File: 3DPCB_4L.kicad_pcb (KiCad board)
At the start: 4 copper layers, 100 x 60 mm, 758 parts, among them IC1 DRV8825, IC2 DRV8825, IC3 DRV8825, IC4 DRV8825, IC5 DRV8825, IC6 MP9943, J10 , J11 , J12 , J13 , J14 , J15 , J16 , J2 , J3 , J4 , J5 , J6 , J7 , J8 , J9 , K1 CONN_3, K2 CONN_3, K3 CONN_3, K4 CONN_3, K5 CONN_3, K6 CONN_3, K7 CONN_3, K8 CONN_3, K9 CONN_3, P1 CONN_8, P11 CONN_3X2, P12 CONN_3X2, P13 CONN_4, P2 CONN_8, P5 CONN_4, P6 CONN_4, P7 CONN_4, P8 CONN_2, P9 CONN_4, U1 CONN_4_LERCHE, U10 MICRO-SD, U11 IX4427, U12 MCP4728, U13 CONN_4_LERCHE, U15 SPST_MOMENTARY, U16 CONN_4_LERCHE, U17 IX4427, U2 SPST_MOMENTARY, U21 CONN_4_LERCHE, U22 CONN_4_LERCHE, U23 MCP4728, U24 IRFH7932, U25 CONN_4_LERCHE, U3 BSS84, U4 CONN_4_LERCHE, U5 IRFH7932, U6 LPC1768_TQFP100, U7 IRFH7932, U8 IRFH7932

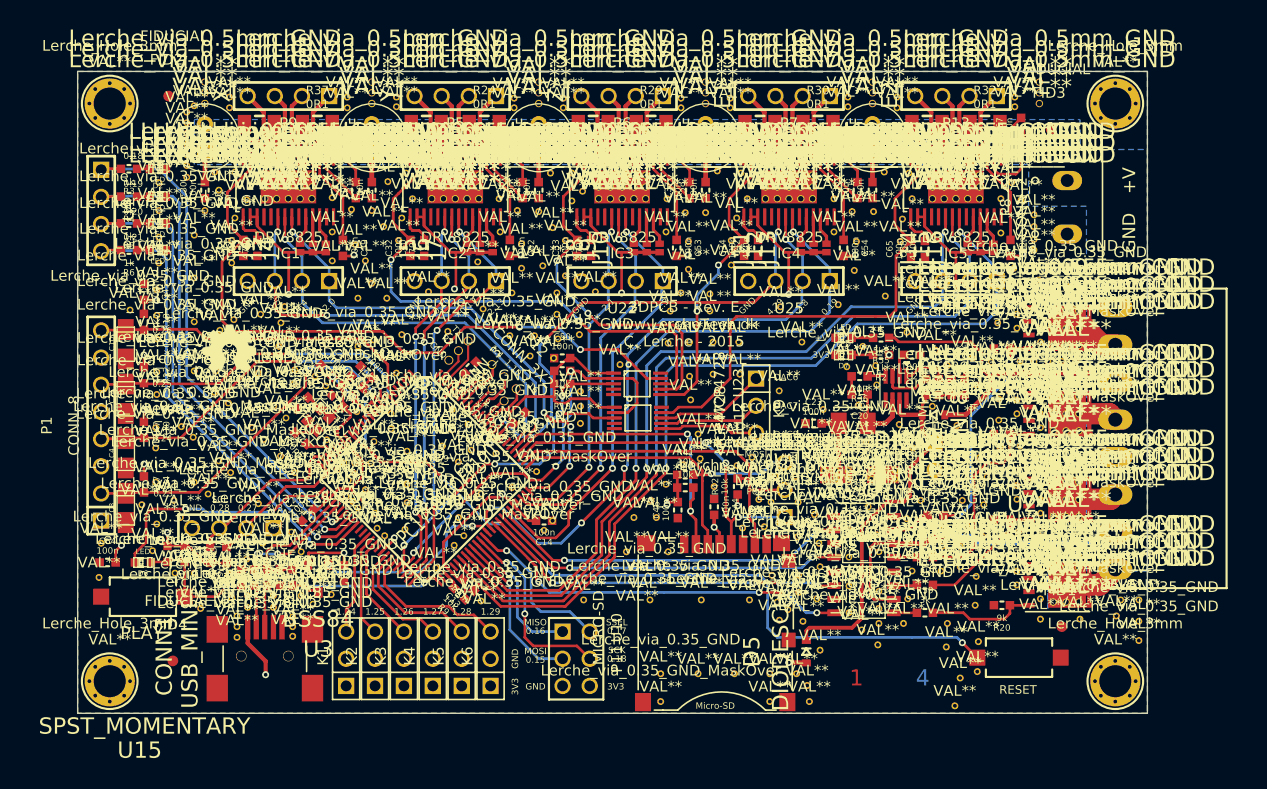
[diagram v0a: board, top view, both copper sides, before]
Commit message: All files added - Hardware is NOT tested yet
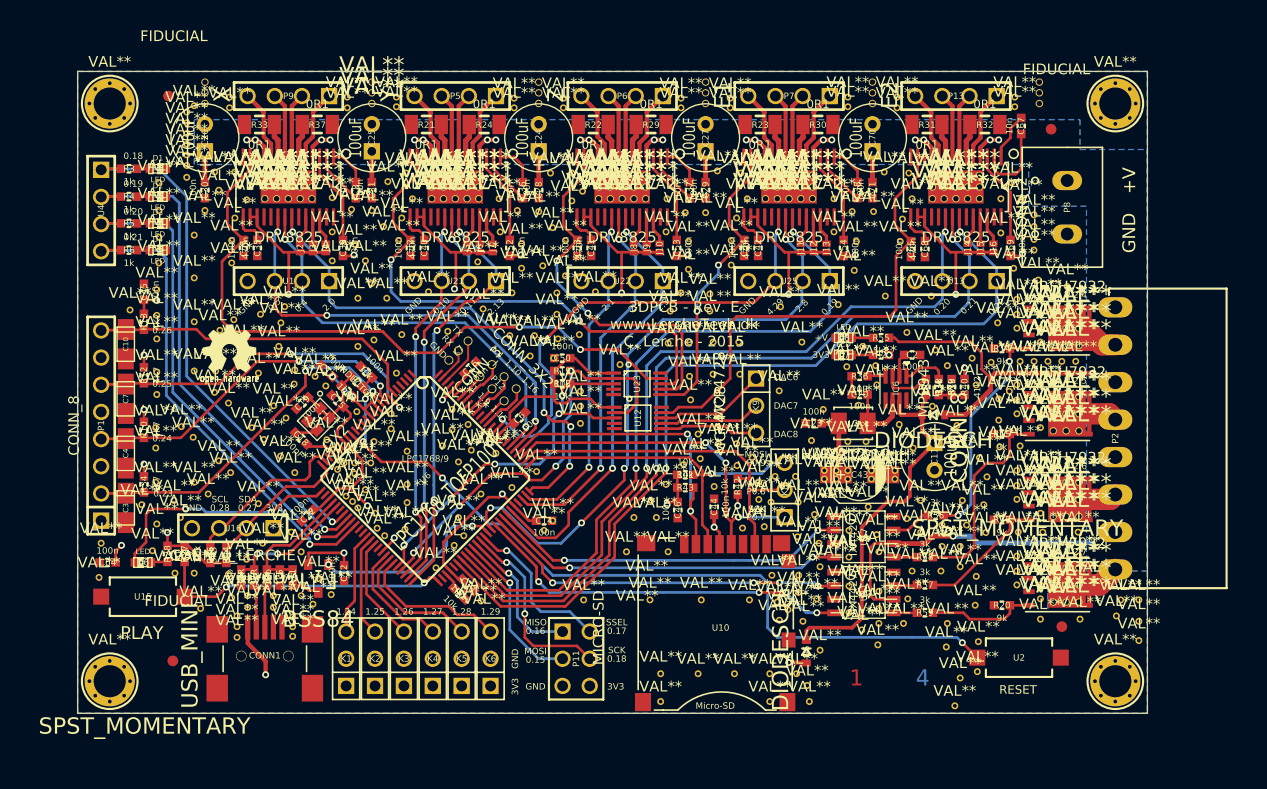
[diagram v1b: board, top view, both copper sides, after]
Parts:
- ? (x21): renamed from Lerche_via_0.5mm_GND; value VAL** -> (none)
- ?: value VAL** -> (none)
- moved ? 5.51 mm to (143.3, 182.8)
- renumbered G*** to ?, Lerche_via_0.5mm_GND to ?, Lerche_via_0.35_GND to ?, Lerche_via_0.35_+12V to ?, Lerche_via_0.35_GND_MaskOver to ?, Lerche_Hole_3mm to ?, FID1 to ?, FID2 to ?, FID3 to ?, FID4 to ?
